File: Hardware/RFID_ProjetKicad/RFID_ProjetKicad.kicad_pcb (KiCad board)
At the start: 2 copper layers, 25 parts, among them J1 TB0011-350-04GR, J2 TB0011-350-04GR, U1 XIAO-ESP32-C6-DIP, U2 CEG006900, U3 MAX3485CSA_T

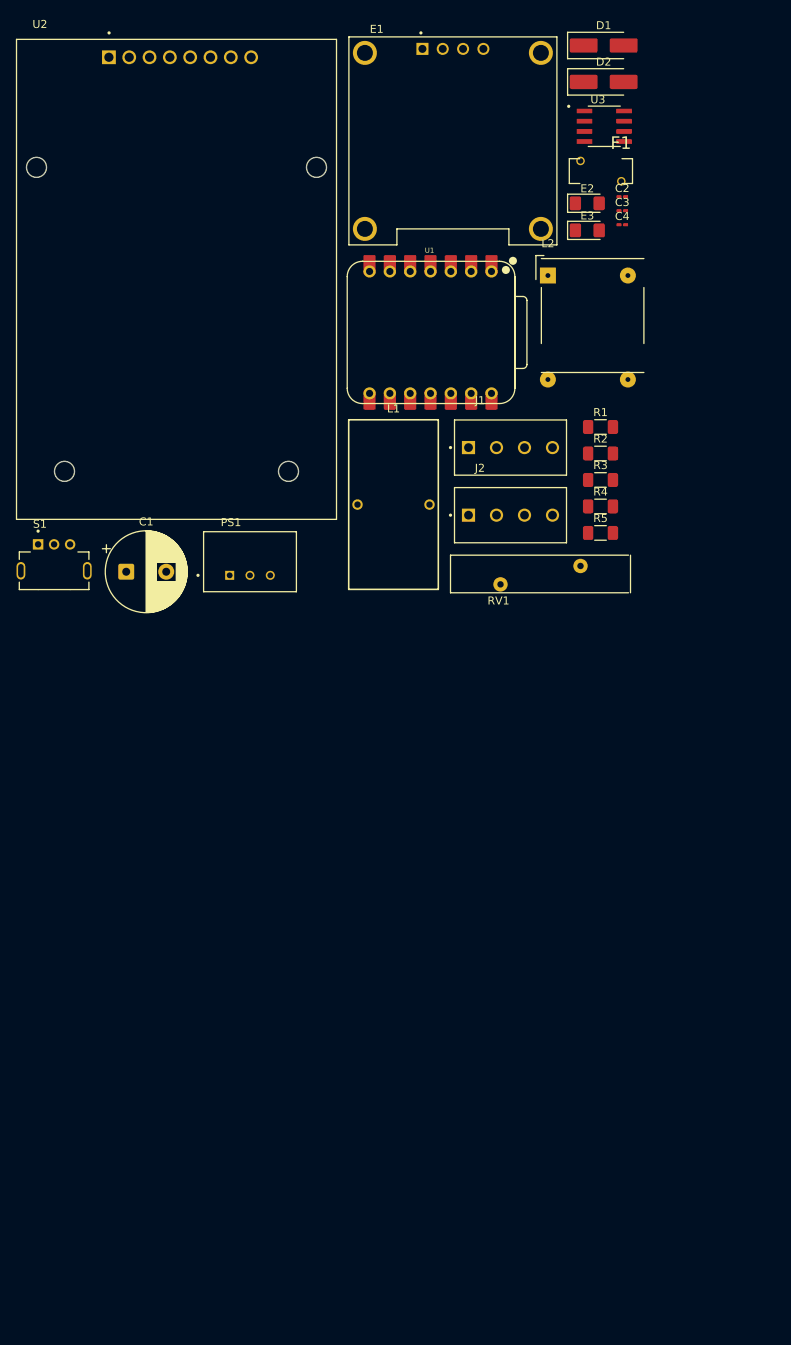
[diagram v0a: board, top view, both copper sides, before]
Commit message: Création du PCB
placement, routage et controle
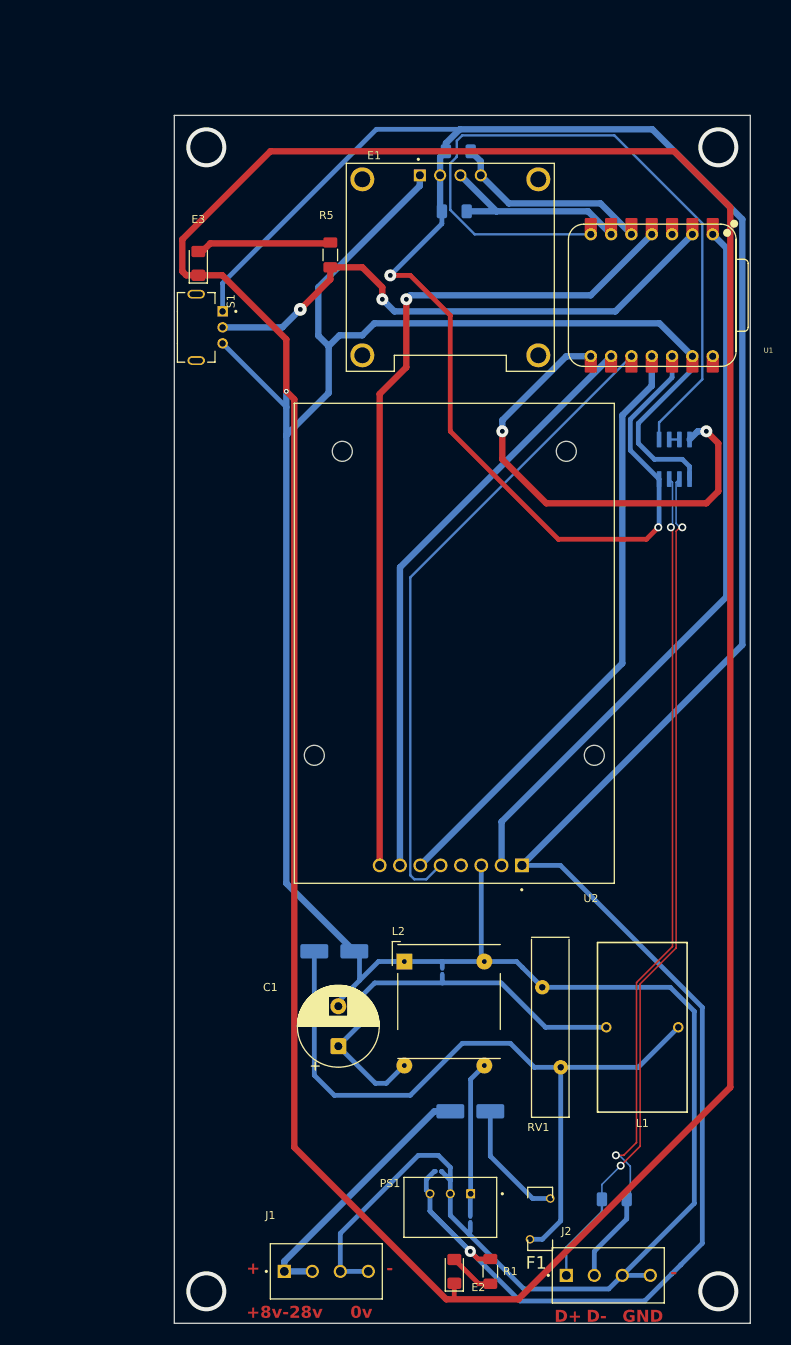
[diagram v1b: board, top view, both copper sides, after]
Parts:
- C2, C3, C4, D1, D2, R2, R3, R4, U3: moved to B.Cu
- L2: value 5 mH -> (none)
- moved E2 134.5 mm to (78.0, 176.0), turned to 90 degrees
- moved D1 134.3 mm to (80.0, 156.0), turned to 180 degrees
- moved F1 131.2 mm to (88.7, 169.4), turned to -90 degrees
- moved C3 127.5 mm to (80.0, 169.5), turned to -90 degrees
- moved C4 120.5 mm to (76.0, 163.5)
- moved D2 113.8 mm to (63.0, 136.0)
- moved R1 106.4 mm to (82.5, 176.0), turned to -90 degrees
- moved J1 105.5 mm to (62.0, 176.0)
- moved C2 99.4 mm to (76.5, 138.5), turned to 90 degrees
- moved J2 95.8 mm to (97.2, 176.5)
- moved R2 93.2 mm to (98.0, 167.0), turned to 180 degrees
- moved L2 87.6 mm to (71.8, 137.3)
- moved PS1 84.5 mm to (77.5, 168.0), turned to 180 degrees
- moved L1 72.4 mm to (101.5, 145.5), turned to 180 degrees
- moved C1 65.0 mm to (63.5, 147.9), turned to 90 degrees
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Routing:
- net GND: track 0.00 -> 749.6 mm, vias 0 -> 1
- net +3V3: track 0.00 -> 394.7 mm, vias 0 -> 3
- net Net-(U1-GPIO21_D3): track 0.00 -> 107.0 mm, vias 0 -> 1
- net /D+: track 0.00 -> 106.4 mm, vias 0 -> 2
- net /D-: track 0.00 -> 106.2 mm, vias 0 -> 2
- net Net-(U1-GPIO16_D6_TX): track 0.00 -> 93.4 mm
- net Net-(U1-GPIO0_A0_D0): track 0.00 -> 92.1 mm
- net +7V à 27.6V: track 0.00 -> 92.0 mm
- net Net-(U1-GPIO20_D9_MISO): track 0.00 -> 81.9 mm
- net Net-(U1-GPIO18_D10_MOSI): track 0.00 -> 76.5 mm
- net Net-(U1-GPIO19_D8_SCK): track 0.00 -> 75.4 mm
- net /SW_COM: track 0.00 -> 70.7 mm, vias 0 -> 2
- net Net-(U1-GPIO17_D7_RX): track 0.00 -> 60.6 mm, vias 0 -> 2
- net Net-(C1-Pad1): track 0.00 -> 53.9 mm
- net +8V à 28V: track 0.00 -> 33.3 mm
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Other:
- board outline added: 72 x 151 mm
- board text added: "+"
- board text added: "+8v-28v"
- board text added: "-"
- board text added: "0v"
- board text added: "D+"
- board text added: "D-"
- board text added: "GND"
